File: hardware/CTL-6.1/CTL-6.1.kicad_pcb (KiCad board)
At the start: 2 copper layers, 107.6 x 45.1 mm, 79 parts, among them J1 Conn_02x16_Top_Bottom, J3 Conn_01x03, J4 Conn_01x03, J5 Conn_02x06_Odd_Even, J6 Conn_01x04, J7 Conn_01x04, K1 G5V-1, Q1 BCX56, Q2 BCX56, Q3 BCX56, Q4 BCX56, Q5 BCX56, Q6 BCX56, SW1 SW_Omron_B3FS, SW2 SW_Omron_B3FS, U1 AMS1117-3.3, U10 OPA365, U2 AMS1117-1.8, U3 OPA365, U5 74LVC1G32, U6 PC817, U7 PC817, U8 USBLC6-2SC6, U9 OPA365

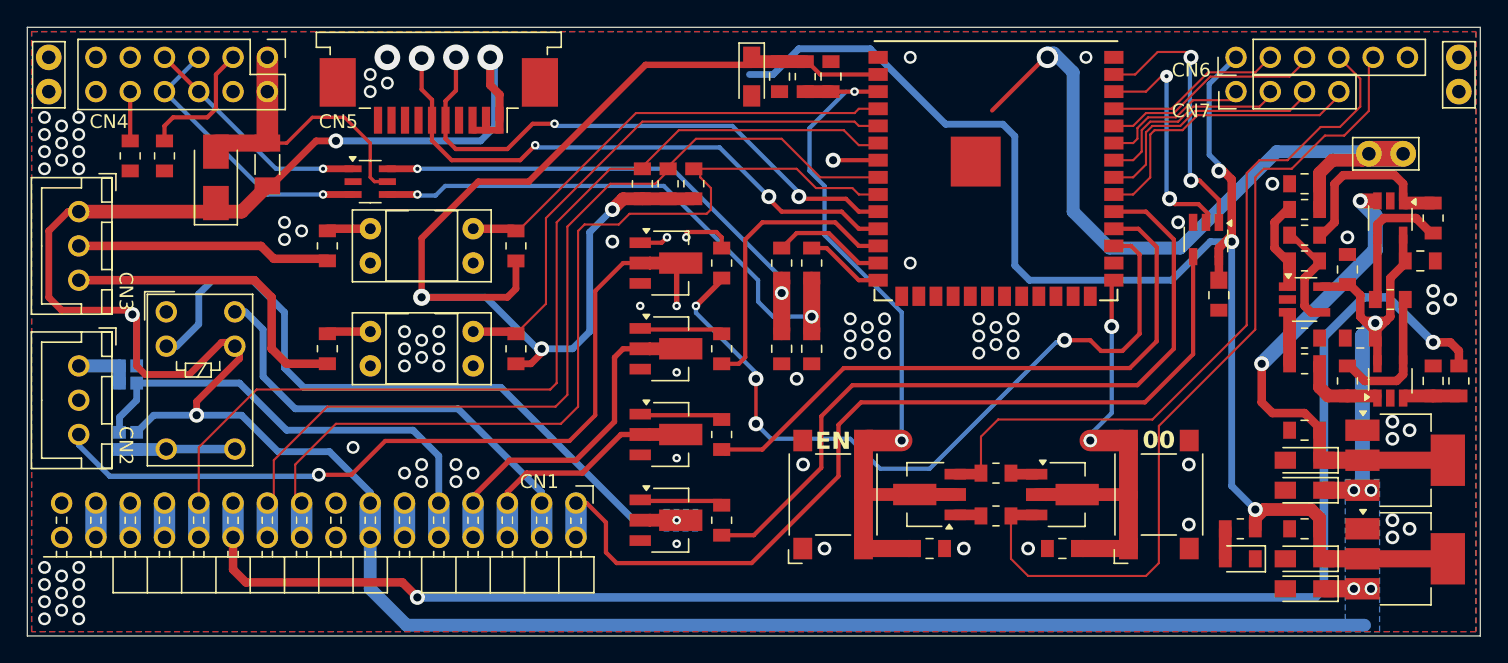
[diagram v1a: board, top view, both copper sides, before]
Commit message: new file:   hardware/CTL-6.0/CTL-6.0-backups/CTL-6.0-2026-06-11_110233.zip 	modified:   hardware/CTL-6.0/CTL-6.0.kicad_prl 	modified:   hardware/CTL-6.0/CTL-6.0.kicad_pro 	deleted:    hardware/CTL-6.1/CTL-6.1-backups/CTL-6.1-2026-05-21_160708.zip 	deleted:    hardware/CTL-6.1/CTL-6.1-backups/CTL-6.1-2026-05-21_163235.zip 	deleted:    hardware/CTL-6.1/CTL-6.1-backups/CTL-6.1-2026-05-22_160447.zip 	deleted:    hardware/CTL-6.1/CTL-6.1-backups/CTL-6.1-2026-05-22_160956.zip 	deleted:    hardware/CTL-6.1/CTL-6.1-backups/CTL-6.1-2026-05-22_162109.zip 	deleted:    hardware/CTL-6.1/CTL-6.1-backups/CTL-6.1-2026-05-22_163223.zip 	deleted:    hardware/CTL-6.1/CTL-6.1-backups/CTL-6.1-2026-05-22_210324.zip 	deleted:    hardware/CTL-6.1/CTL-6.1-backups/CTL-6.1-2026-05-25_112244.zip 	new file:   hardware/CTL-6.1/CTL-6.1-backups/CTL-6.1-2026-06-11_110530.zip 	new file:   hardware/CTL-6.1/CTL-6.1-backups/CTL-6.1-2026-06-11_110702.zip 	new file:   hardware/CTL-6.1/CTL-6.1-backups/CTL-6.1-2026-06-11_111015.zip 	new file:   hardware/CTL-6.1/CTL-6.1-backups/CTL-6.1-2026-06-11_111525.zip 	new file:   hardware/CTL-6.1/CTL-6.1-backups/CTL-6.1-2026-06-11_112032.zip 	new file:   hardware/CTL-6.1/CTL-6.1-backups/CTL-6.1-2026-06-11_112817.zip 	new file:   hardware/CTL-6.1/CTL-6.1-backups/CTL-6.1-2026-06-11_113247.zip 	new file:   hardware/CTL-6.1/CTL-6.1-backups/CTL-6.1-2026-06-11_115705.zip 	new file:   hardware/CTL-6.1/CTL-6.1-backups/CTL-6.1-2026-06-11_115856.zip 	modified:   hardware/CTL-6.1/CTL-6.1.kicad_pcb 	modified:   hardware/CTL-6.1/CTL-6.1.kicad_prl 	modified:   hardware/CTL-6.1/CTL-6.1.kicad_pro 	modified:   hardware/CTL-6.1/CTL-6.1.kicad_sch 	new file:   hardware/CTL-6.1/~CTL-6.1.kicad_pcb.lck 	new file:   hardware/CTL-6.1/~CTL-6.1.kicad_pro.lck 	new file:   hardware/CTL-6.1/~CTL-6.1.kicad_sch.lck
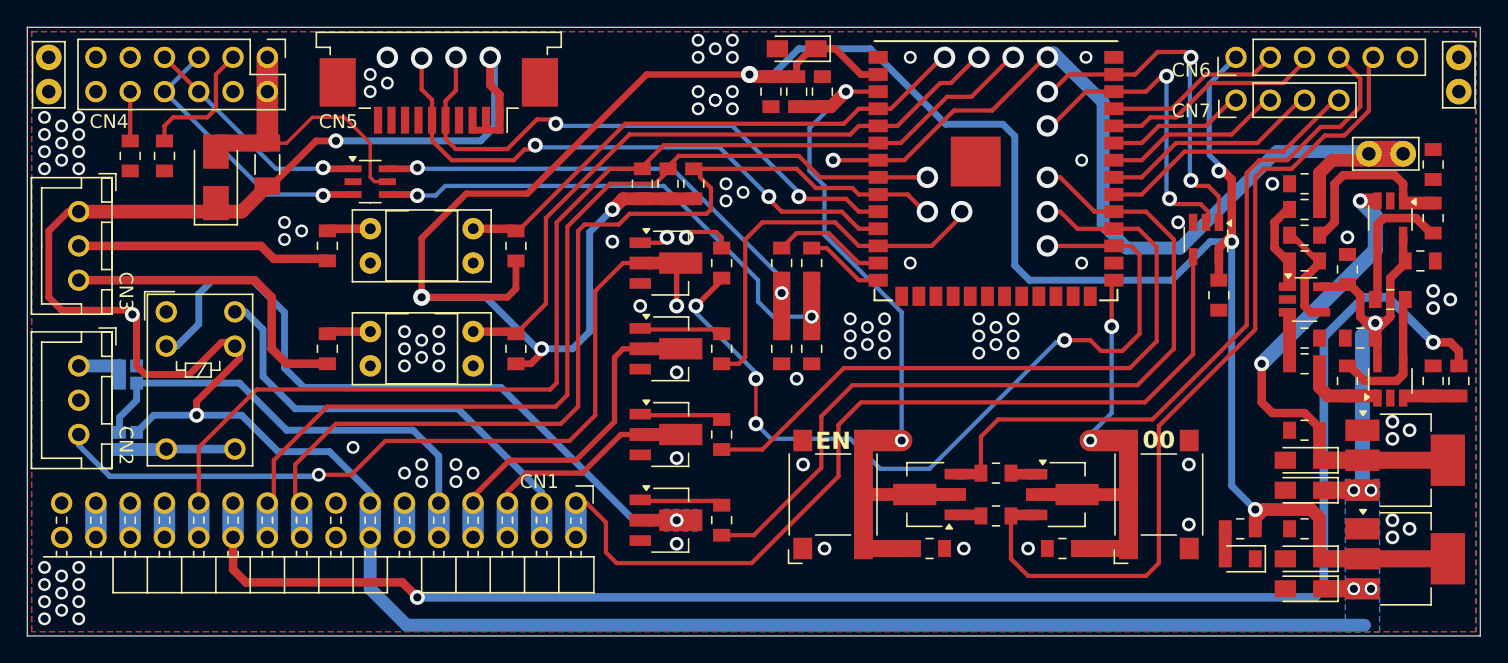
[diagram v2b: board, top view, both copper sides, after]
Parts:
- added R30: 3.3kΩ, Resistor_SMD:R_0805_2012Metric_Pad1.20x1.40mm_HandSolder, F.Cu at (139.1, 72.9)
- R29: value 10kΩ -> 1.8kΩ
- moved C19 9.63 mm to (148.6, 71.4), turned to -90 degrees
- moved C10 3.92 mm to (101.4, 62.9), turned to 180 degrees
- moved C11 1.28 mm to (99.5, 66.0)
- moved C9 1.28 mm to (103.3, 66.0)
- moved R16 1.28 mm to (101.4, 66.0)
- moved J7 0.63 mm to (134.0, 66.7)
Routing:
- net /OPTO: track 74.1 -> 85.8 mm, vias 0 -> 1
- net /SEN-COAG: track 40.1 -> 49.4 mm, vias 0 -> 1
- net /REM: track 58.0 -> 67.2 mm
- net /CTL-RLY-A.1: track 21.7 -> 29.2 mm, vias 0 -> 1
- net /SEN-CUT: track 33.5 -> 40.0 mm, vias 0 -> 1
- net /PWM.01: track 17.5 -> 23.6 mm, vias 2 -> 3
- net /CTL-PWM-EN: track 54.8 -> 60.8 mm, vias 0 -> 1
- net /PWM.00: track 20.1 -> 25.7 mm, vias 2 -> 3
- net /CTL-RLY-A.2: track 46.7 -> 52.2 mm, vias 0 -> 1
- net /CTL-BUZZ: track 56.3 -> 61.2 mm, vias 4 -> 5
- net /MSD1: track 69.6 -> 73.8 mm, vias 0 -> 1
- net /MSD2: track 69.5 -> 72.1 mm, vias 0 -> 1
- net +3.3V: track 193.2 -> 195.4 mm, vias 6 -> 7
- net /TCK: track 21.4 -> 19.5 mm
- net /TDO: track 17.9 -> 16.5 mm
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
